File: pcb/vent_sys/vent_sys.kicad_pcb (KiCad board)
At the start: 2 copper layers, 88.9 x 53.3 mm, 19 parts, among them J1 Screw_Terminal_01x02, J2 Screw_Terminal_01x02, Q1 BT138-600, U1 PC817, U2 stm32f103c8t6-module-china, U3 MOC3021M, U4 RA-02

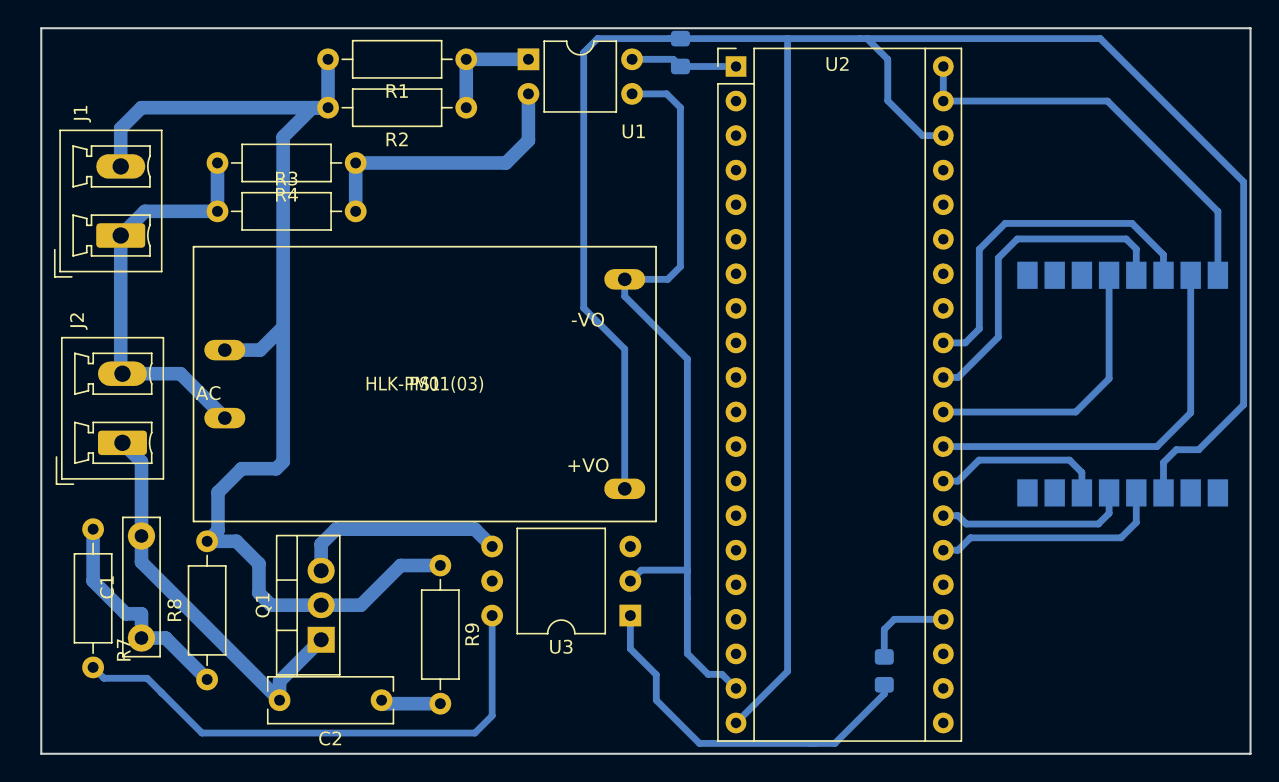
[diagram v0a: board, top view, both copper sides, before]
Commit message: final
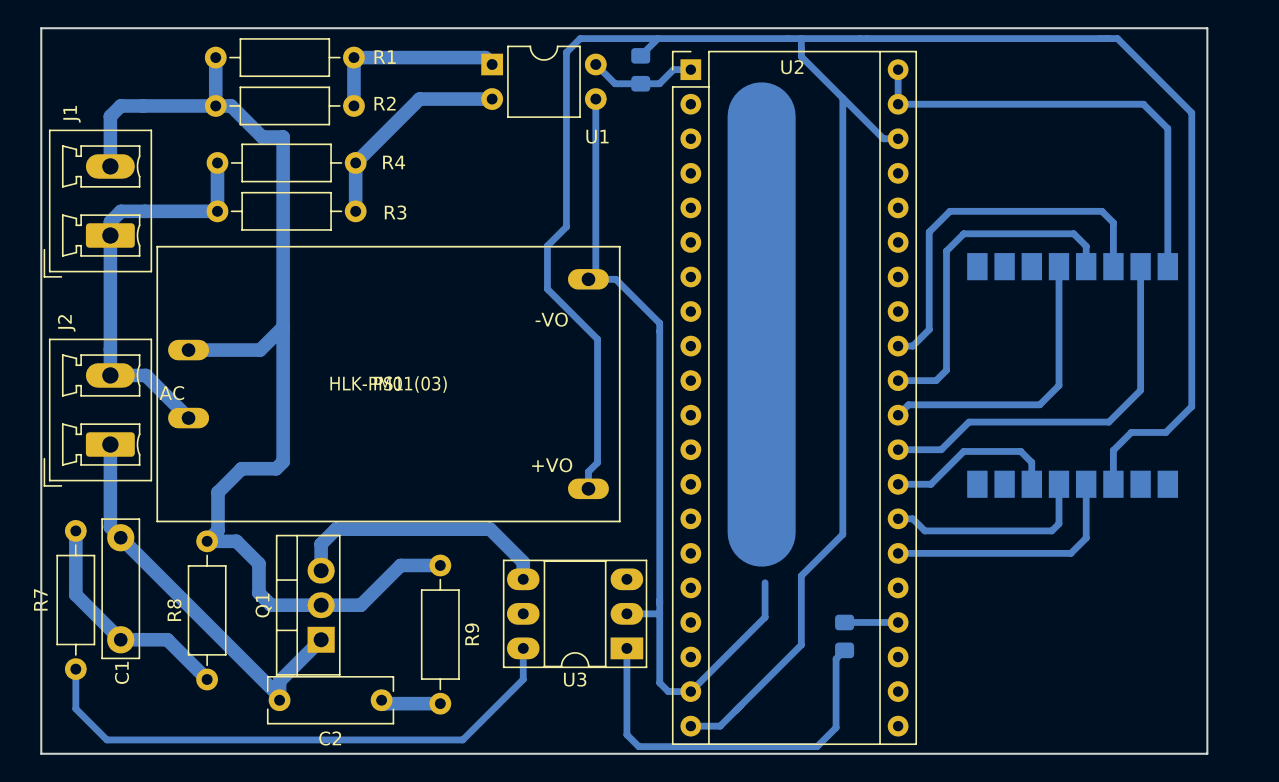
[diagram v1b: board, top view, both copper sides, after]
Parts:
- U3: footprint Package_DIP:DIP-6_W10.16mm -> Package_DIP:DIP-6_W7.62mm_Socket_LongPads
- moved R1 8.26 mm to (82.7, 51.7)
- moved R2 8.26 mm to (82.7, 55.2)
- moved R6 3.86 mm to (118.7, 94.2)
- moved U4 3.74 mm to (135.5, 75.1)
- moved U2 3.33 mm to (107.4, 52.6)
- moved R5 3.19 mm to (103.8, 52.6)
- moved U1 2.69 mm to (92.8, 52.2)
- moved PS1 2.67 mm to (85.2, 75.7)
- moved U3 2.43 mm to (102.7, 95.1)
- moved C1 1.53 mm to (65.5, 94.5)
- moved R7 1.28 mm to (62.2, 96.6)
- moved J2 0.90 mm to (64.8, 80.1)
- moved J1 0.76 mm to (64.8, 64.8)
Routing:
- net (no net): track 0.00 -> 30.6 mm
- net Net-(R1-Pad1): track 8.13 -> 13.9 mm
- net Net-(R3-Pad2): track 20.4 -> 15.5 mm
- net VCC: track 175.1 -> 179.9 mm
- net Net-(Q1-Pad3): track 15.5 -> 19.5 mm
- net GND: track 58.7 -> 62.0 mm
- net Net-(R6-Pad1): track 6.67 -> 3.94 mm
- net /L: track 86.5 -> 83.9 mm
- net Net-(U2-Pad39): track 30.8 -> 33.3 mm
- net /MOSI: track 25.7 -> 27.7 mm
- net Net-(R7-Pad1): track 39.4 -> 40.9 mm
- net /MISO: track 24.0 -> 25.3 mm
- net /nIRQ: track 14.3 -> 15.3 mm
- net /Reset: track 17.2 -> 18.2 mm
- net Net-(R6-Pad2): track 27.6 -> 28.6 mm
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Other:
- board size 88.9 x 53.3 mm -> 85.7 x 53.3 mm
